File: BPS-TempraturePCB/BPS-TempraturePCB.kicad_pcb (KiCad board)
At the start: 2 copper layers, 70.6 x 66.7 mm, 40 parts, among them J1 Conn_01x24_Female, J2 TEMPSPIANALYZER, U2 LM321, U3 ADS7953SBDBT, U5 REF4132B25DBVR

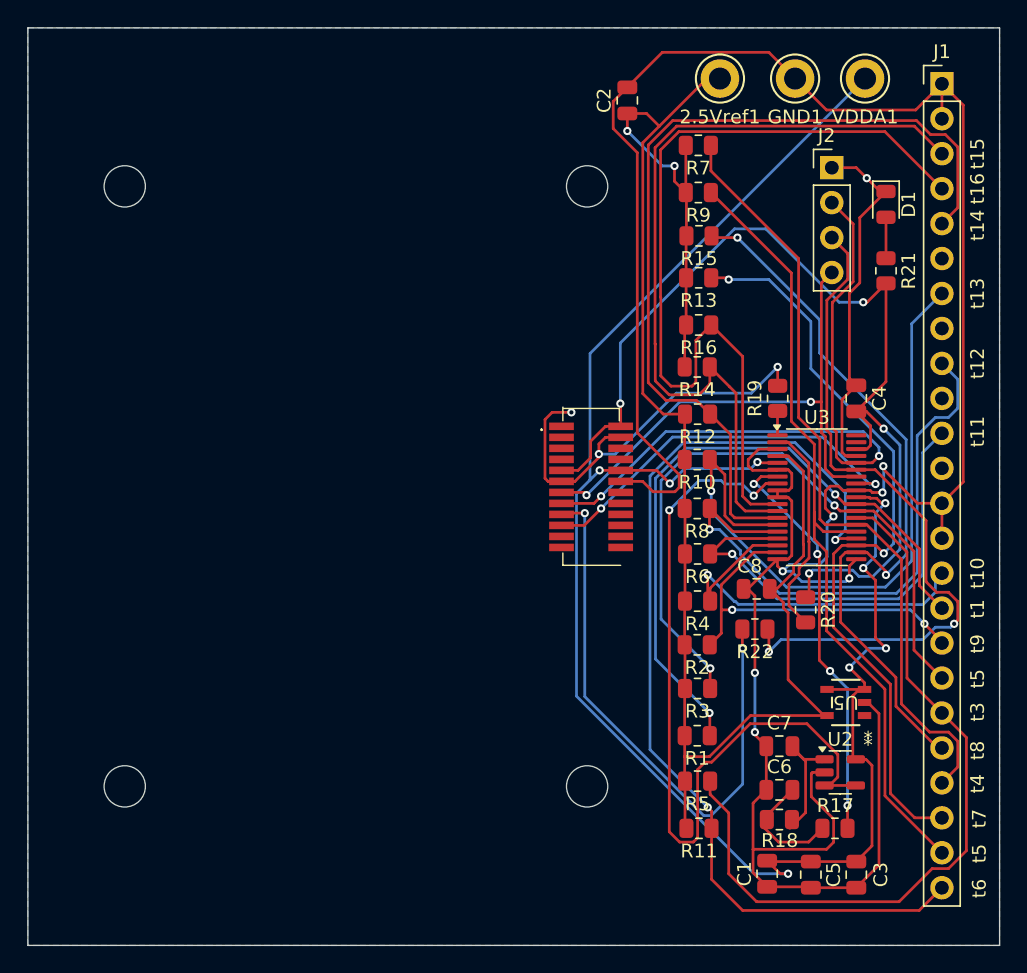
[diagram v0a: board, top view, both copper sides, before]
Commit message: Redid routing to be better.
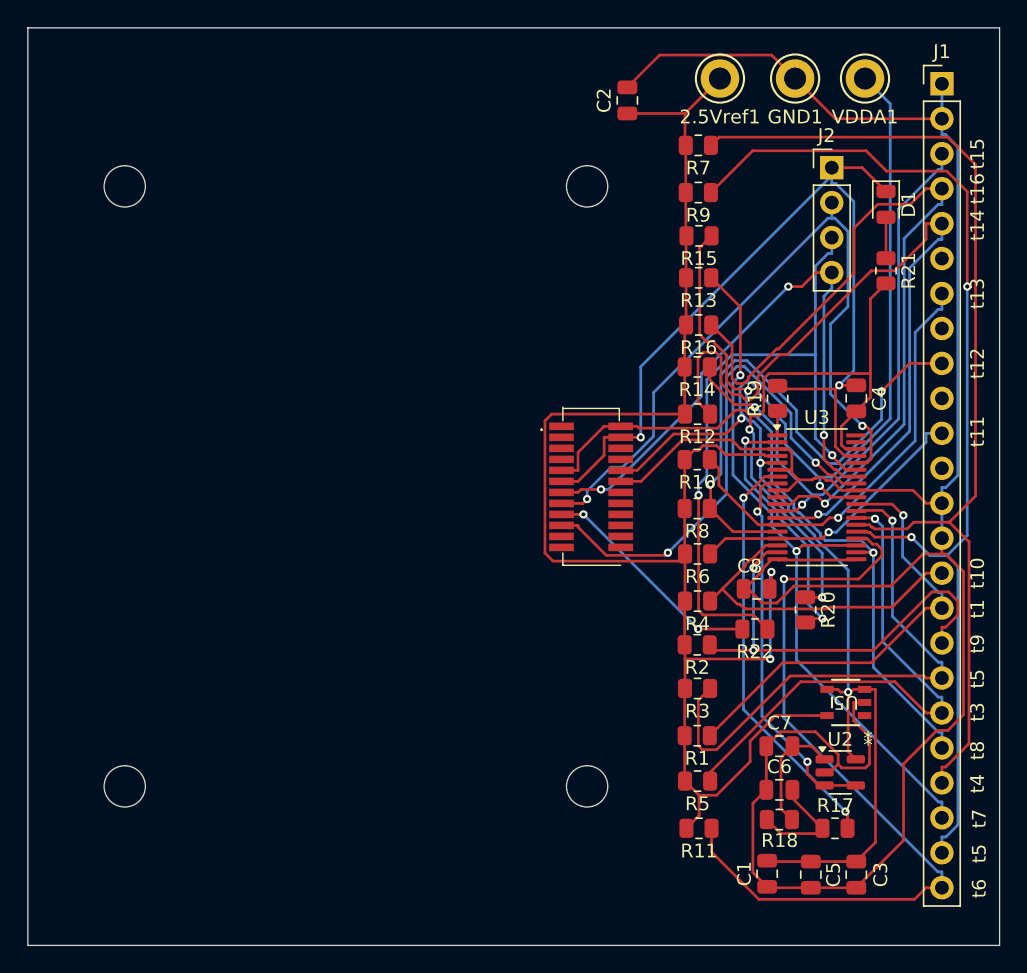
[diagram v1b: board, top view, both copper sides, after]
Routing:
- net /ADCIN: track 58.0 -> 27.6 mm
- net Net-(U4-SPI1_MOSI): track 42.3 -> 16.6 mm
- net GNDA: track 204.4 -> 180.3 mm, vias 7 -> 0
- net VDDA: track 134.5 -> 111.9 mm, vias 8 -> 4
- net /temp13: track 50.4 -> 31.8 mm
- net /temp5: track 59.8 -> 78.1 mm, vias 0 -> 2
- net /temp4: track 56.8 -> 74.7 mm
- net /temp3: track 55.1 -> 38.8 mm, vias 0 -> 1
- net /temp1: track 48.4 -> 32.6 mm, vias 2 -> 1
- net +3.3V: track 73.5 -> 59.0 mm, vias 4 -> 2
- net /temp15: track 59.1 -> 45.5 mm, vias 0 -> 2
- net /temp6: track 71.5 -> 58.1 mm, vias 2 -> 1
- net /temp11: track 33.7 -> 20.9 mm
- net /SPI1_NSS: track 28.3 -> 37.7 mm
- net GND: track 57.4 -> 66.3 mm, vias 4 -> 2
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- removed copper zone on B.Cu, net GND
